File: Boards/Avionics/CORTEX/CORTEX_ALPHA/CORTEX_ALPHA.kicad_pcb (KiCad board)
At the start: 2 copper layers, 97.1 x 83 mm, 22 parts, among them J1 Conn_01x06_Pin, J2 Screw_Terminal_01x02, J3 1200700164, J4 Conn_01x06_Pin, U2 E28-2G4M27S_LoRa, U3 MAX485_MODULE_5V_LOGIC_TLL_TO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, U4 NUCLEO-G431KB

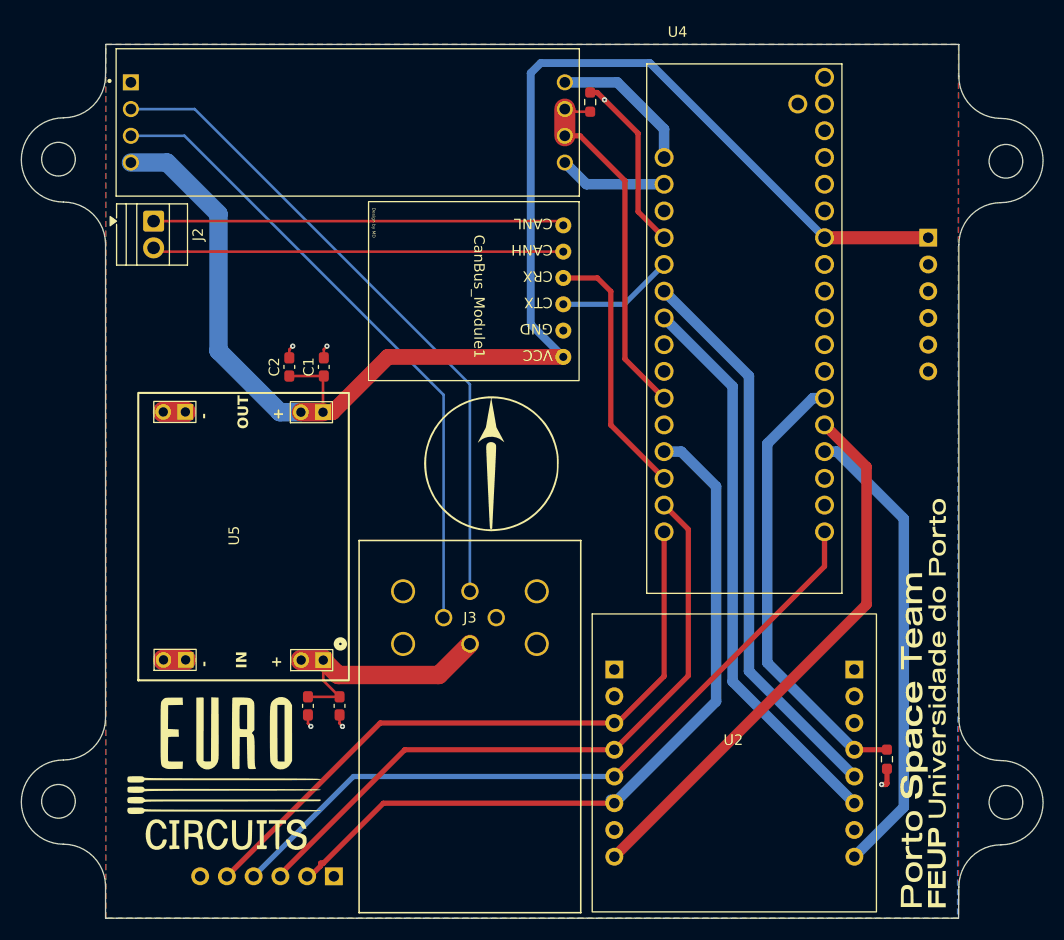
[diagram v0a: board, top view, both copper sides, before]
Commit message: changes cortex
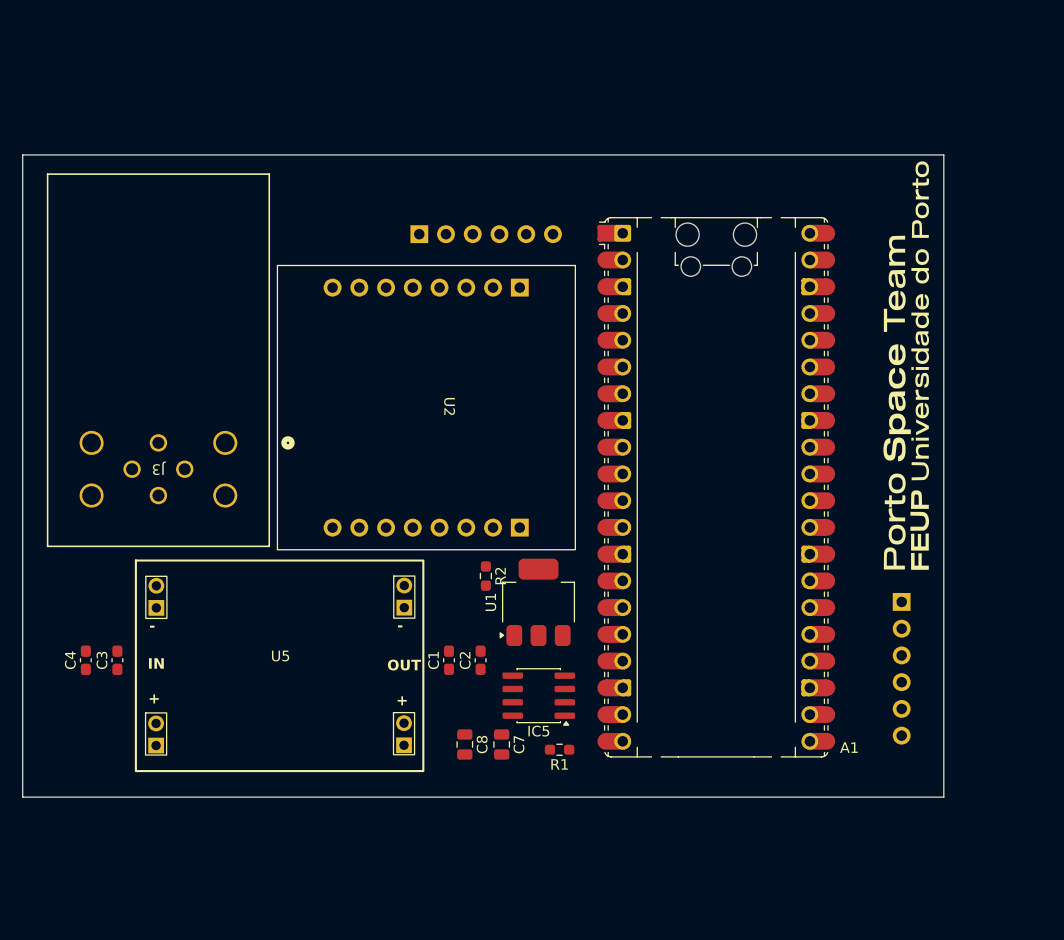
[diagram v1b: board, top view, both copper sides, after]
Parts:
- removed CanBus_Module1: ~, CORTEX:Canbus
- removed J2: Screw_Terminal_01x02, TerminalBlock:TerminalBlock_Xinya_XY308-2.54-2P_1x02_P2.54mm_Horizontal
- removed REF** (x4): MountingHole_3.2mm_M3_DIN965, MountingHole:MountingHole_3.2mm_M3_DIN965
- removed U3: MAX485_MODULE_5V_LOGIC_TLL_TO_RS-485_CONVERTER, MAX485_MODULE_5V_LOGIC_TLL_TO_RS-485_CONVERTER:MODULE_MAX485_MODULE_5V_LOGIC_TLL_TO_RS-485_CONVERTER
- removed U4: NUCLEO-G431KB, NUCLEO_G431KB:MODULE_NUCLEO-G431KB
- added A1: RaspberryPi_Pico, Module:RaspberryPi_Pico_Common_Unspecified, F.Cu at (157.9, 100.6)
- added C7: 0.1uF, Capacitor_SMD:C_0805_2012Metric, F.Cu at (137.5, 125.0)
- added C8: C_Small, Capacitor_SMD:C_0805_2012Metric, F.Cu at (134.0, 125.0)
- added IC5: SP3485CN-L_TR, Package_SO:SOIC-8_3.9x4.9mm_P1.27mm, F.Cu at (141.0, 120.4)
- added U1: LD1117S33TR_SOT223, Package_TO_SOT_SMD:SOT-223-3_TabPin2, F.Cu at (141.0, 111.5)
- G*** (x2): moved to B.Cu
- moved R1 61.6 mm to (143.0, 125.5), turned to 180 degrees
- moved J1 61.5 mm to (129.7, 76.5), turned to -90 degrees
- moved U2 44.4 mm to (130.5, 93.0), turned to -90 degrees
- moved R2 41.9 mm to (136.0, 109.0)
- moved G*** 41.4 mm to (101.0, 77.0), turned to 180 degrees
- moved J3 35.2 mm to (104.9, 96.4), turned to 180 degrees
- moved J4 34.7 mm to (175.5, 111.5)
- moved C2 33.3 mm to (135.5, 117.0)
- moved G*** 32.1 mm to (176.0, 89.0)
- moved C1 30.3 mm to (132.5, 117.0)
- moved C3 21.5 mm to (101.0, 117.0), turned to 90 degrees
- moved C4 21.5 mm to (98.0, 117.0), turned to 90 degrees
- moved U5 12.6 mm to (116.5, 117.1), turned to 0 degrees
- moved G*** 11.7 mm to (116.5, 117.5), turned to 180 degrees
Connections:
- J1 pad 2: /CS -> /SD_CS
- U2 pad 6: /CS -> /RADIO_CS
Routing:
- net +5V: track 140.7 -> 0.00 mm
- net /CS: track 73.1 -> 0.00 mm
- net /CLK: track 69.7 -> 0.00 mm
- net /MOSI: track 63.9 -> 0.00 mm
- net /MISO: track 63.1 -> 0.00 mm
- net /RS_A: track 62.7 -> 0.00 mm
- net /RS_B: track 61.1 -> 0.00 mm
- net /ANT_BUSY: track 53.6 -> 0.00 mm
- net /ANT_NRESET: track 53.6 -> 0.00 mm
- net /ANT_RX_EN: track 52.6 -> 0.00 mm
- net /ANT_TX_EN: track 44.2 -> 0.00 mm
- net /ANT_DIO1: track 42.8 -> 0.00 mm
- net Net-(CanBus_Module1-CANL): track 39.1 -> 0.00 mm
- net Net-(CanBus_Module1-CANH): track 39.1 -> 0.00 mm
- net /RS_ENABLE: track 35.6 -> 0.00 mm
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- removed copper zone on F.Cu, net +3.3V
- removed copper zone on B.Cu, net GND
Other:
- board size 97.1 x 83 mm -> 87.5 x 61 mm
- board text removed: "CORTEX"
